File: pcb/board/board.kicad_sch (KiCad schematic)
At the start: 132 parts, among them J1 (A) USB_C_Receptacle_USB2.0_1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, J10 OLED_128x32, J11 LCD_128x160, J12 AudioJack3, J13 Conn_01x02, J14 Micro_SD_Card, J15 Conn_01x03, J16 Conn_01x06, J17 Conn_01x03, J18 Conn_01x03, J19 Conn_01x03, J2 (B) USB_C_Receptacle_USB2.0_1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, J20 Conn_01x04, J21 Conn_01x04, J22 Conn_01x05, J23 Conn_01x05, J24 Conn_01x05, J25 Conn_01x02, J3 (C) USB_C_Receptacle_USB2.0_1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, J4 Conn_01x03, J5 Conn_01x03, J6 Conn_01x04, J7 Conn_01x07, J8 Conn_01x04, J9 Conn_01x02, SW1 SW_Push, SW2 SW_Push, SW3 Switch, SW4 Switch, SW5 Switch, SW6 RotaryEncoder_Switch, U1 RP2040, U2 NCP1117-3.3_SOT223, U3 W25Q16JVZPIQ TR, U4 NCP1117-3.3_SOT223, U5 RP2040, U6 W25Q16JVZPIQ TR, U7 PCM5101A, U8 TLV70033_SOT23-5, U9 TPA6132A2RTE, Y1 12MHz, Y2 12MHz

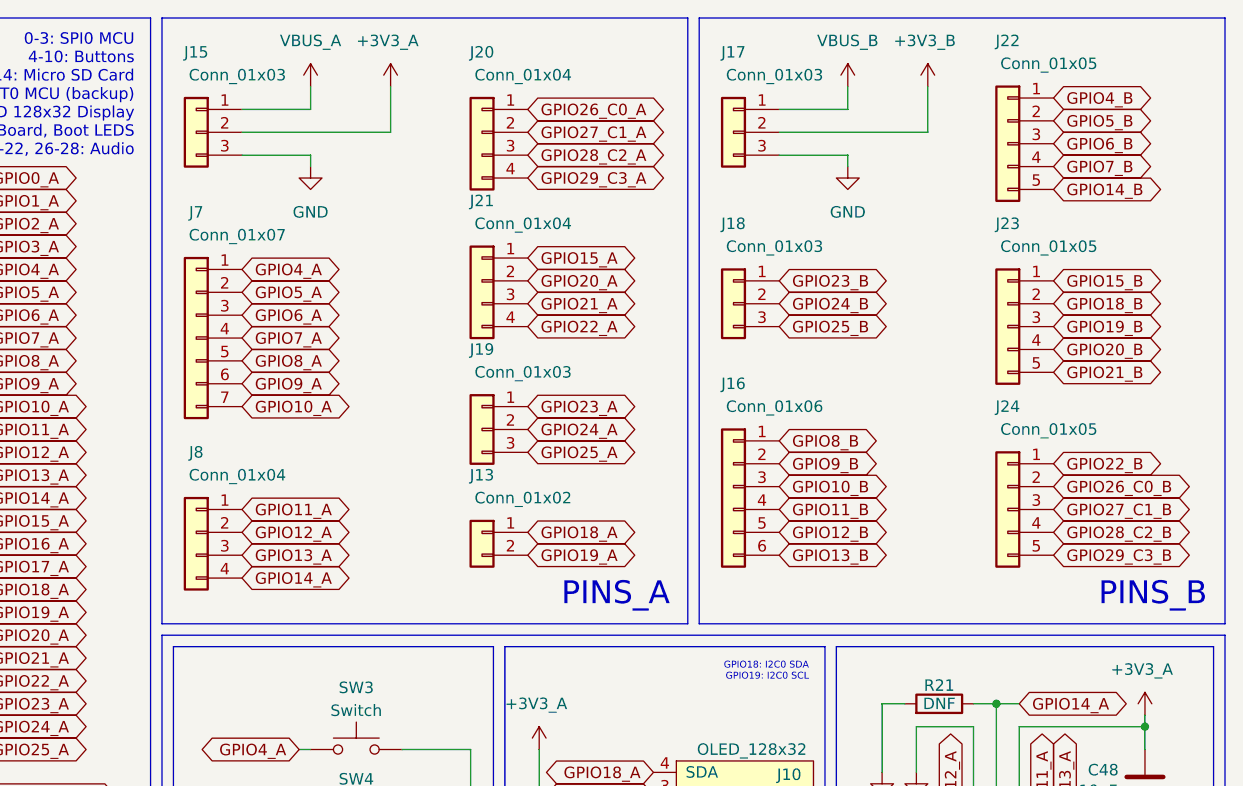
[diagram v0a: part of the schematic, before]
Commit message: leds and more connections!
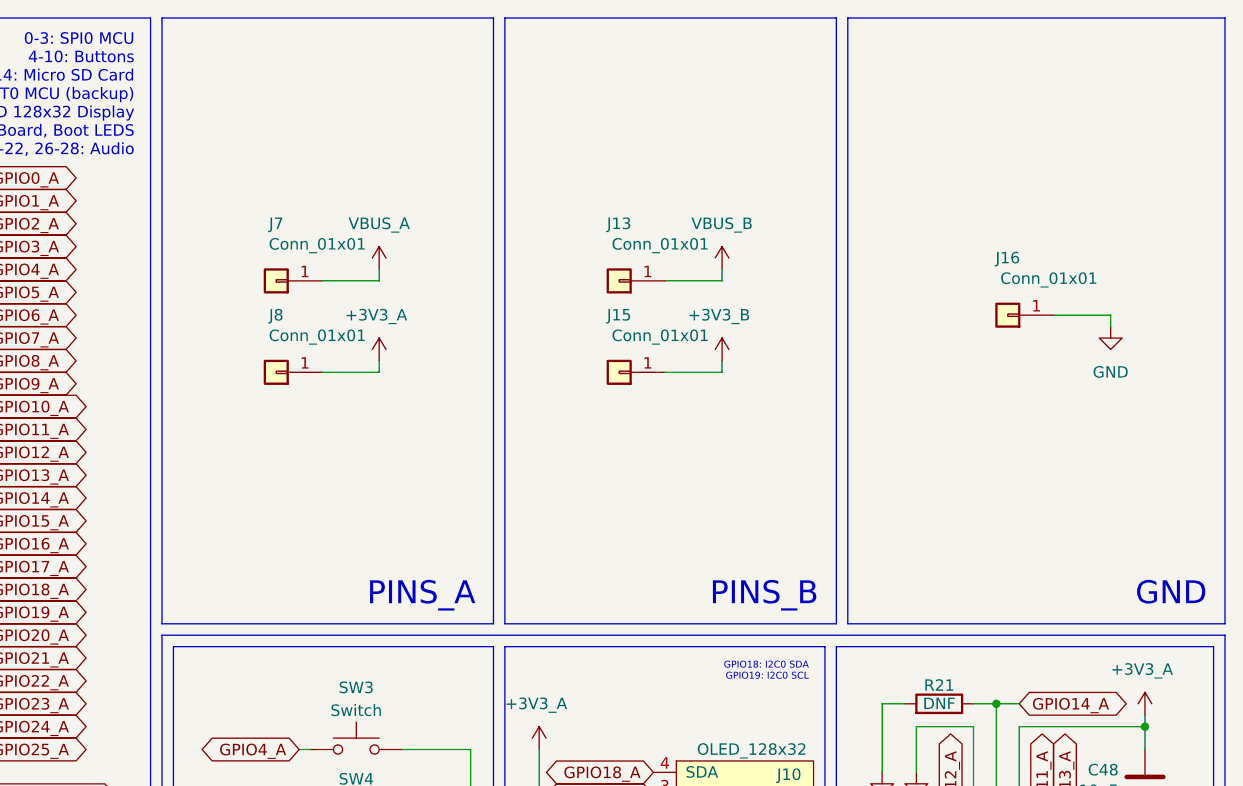
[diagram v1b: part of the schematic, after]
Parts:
- removed J13: Conn_01x02, Connector_PinHeader_2.54mm:PinHeader_1x02_P2.54mm_Vertical, symbol Connector_Generic:Conn_01x02
- removed J15, J17, J18, J19: Conn_01x03, Connector_PinHeader_2.54mm:PinHeader_1x03_P2.54mm_Vertical, symbol Connector_Generic:Conn_01x03
- removed J16: Conn_01x06, Connector_PinHeader_2.54mm:PinHeader_1x06_P2.54mm_Vertical, symbol Connector_Generic:Conn_01x06
- removed J20, J21, J8: Conn_01x04, Connector_PinHeader_2.54mm:PinHeader_1x04_P2.54mm_Vertical, symbol Connector_Generic:Conn_01x04
- removed J22, J23, J24: Conn_01x05, Connector_PinHeader_2.54mm:PinHeader_1x05_P2.54mm_Vertical, symbol Connector_Generic:Conn_01x05
- removed J7: Conn_01x07, Connector_PinHeader_2.54mm:PinHeader_1x07_P2.54mm_Vertical, symbol Connector_Generic:Conn_01x07
- added J13, J7: Conn_01x01, TestPoint:TestPoint_Pad_1.0x1.0mm, symbol Connector_Generic:Conn_01x01
- added J15, J16, J8: Conn_01x01, Connector_PinHeader_2.54mm:PinHeader_1x01_P2.54mm_Vertical, symbol Connector_Generic:Conn_01x01
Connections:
- net +3V3_A: now also J8.1 (Pin_1)
- net +3V3_B: now also J15.1 (Pin_1)
- net GND: now also J16.1 (Pin_1)
- net VBUS_A: now also J7.1 (Pin_1)
- net VBUS_B: now also J13.1 (Pin_1)

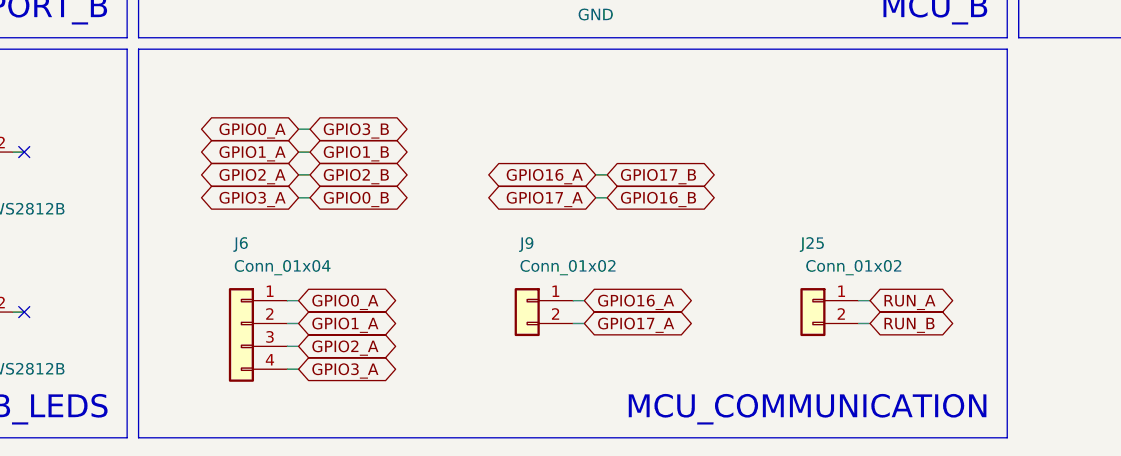
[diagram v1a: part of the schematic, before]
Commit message: 08192026 - starting to wrap up pcb work!
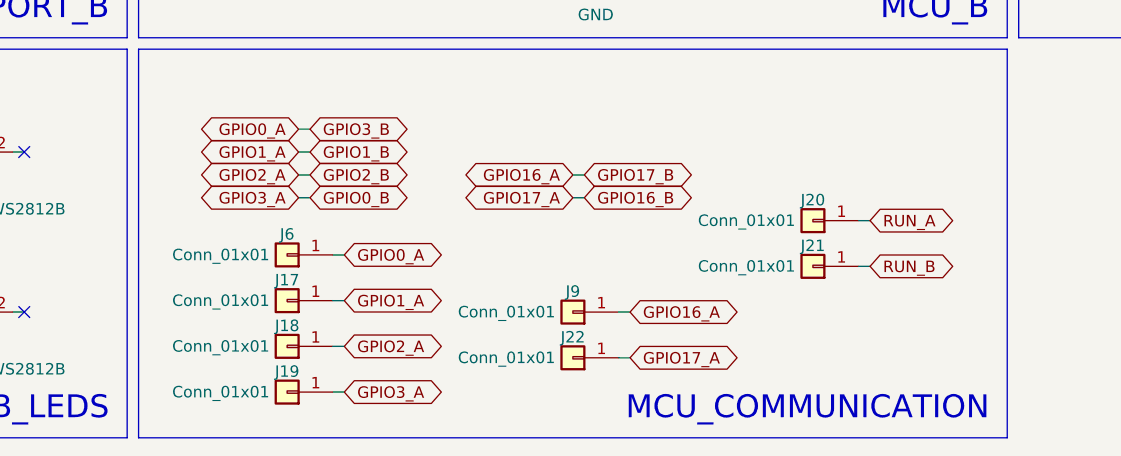
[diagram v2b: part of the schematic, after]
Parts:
- removed J25, J9: Conn_01x02, Connector_PinHeader_2.54mm:PinHeader_1x02_P2.54mm_Vertical, symbol Connector_Generic:Conn_01x02
- removed J6: Conn_01x04, Connector_PinHeader_2.54mm:PinHeader_1x04_P2.54mm_Vertical, symbol Connector_Generic:Conn_01x04
- added J17, J18, J19, J20, J21, J22, J6, J9: Conn_01x01, TestPoint:TestPoint_Pad_D1.0mm, symbol Connector_Generic:Conn_01x01
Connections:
- net GPIO0_A: now also J6.1 (Pin_1)
- net GPIO0_B: now also J19.1 (Pin_1)
- net GPIO16_A: now also J9.1 (Pin_1)
- net GPIO16_B: now also J22.1 (Pin_1)
- net GPIO1_A: now also J17.1 (Pin_1)
- net GPIO2_A: now also J18.1 (Pin_1)
- net RUN_A: now also J20.1 (Pin_1)
- net RUN_B: now also J21.1 (Pin_1)

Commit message: 08232026 - exporting and back to again
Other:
- title: River Board -> River Board Schematic
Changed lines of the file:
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@@
 	(paper "A3")
 	(title_block
-		(title "River Board")
+		(title "River Board Schematic")
+		(date "2026-08-23")
 		(rev "1.0")
 		(company "HenryLi-0")
